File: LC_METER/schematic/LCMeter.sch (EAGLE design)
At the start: 164 parts, among them IC1 74HC595, IC2 74HC595, IC3 74HC595, IC4 74HC595, IC5 74HC595, IC6 MEGA8535, J10 0, J11 0, J123 0, J2 0, J3 0, J4 0, J5 0, J6 0, J7 0, J8 0, J9 0, Q2 12MHz, T1 BC847, T2 BC847, T3 BC857, T4 BC857, T5 BC847, T6 BC847, T7 BC847, U15 LM324, X1 C_X, X4 L_X, X5 USB_B, X6 USB_MICRO

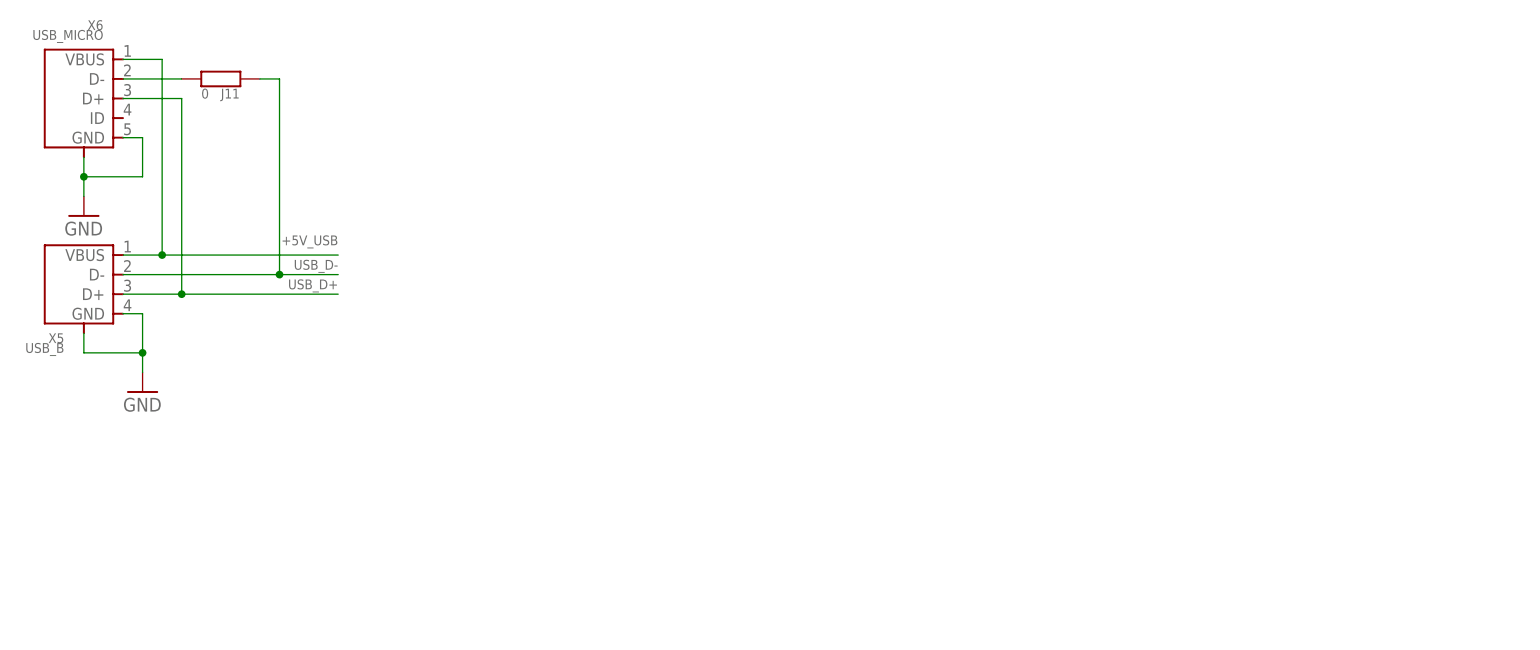
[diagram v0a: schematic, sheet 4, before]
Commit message: LCMeter Another changes
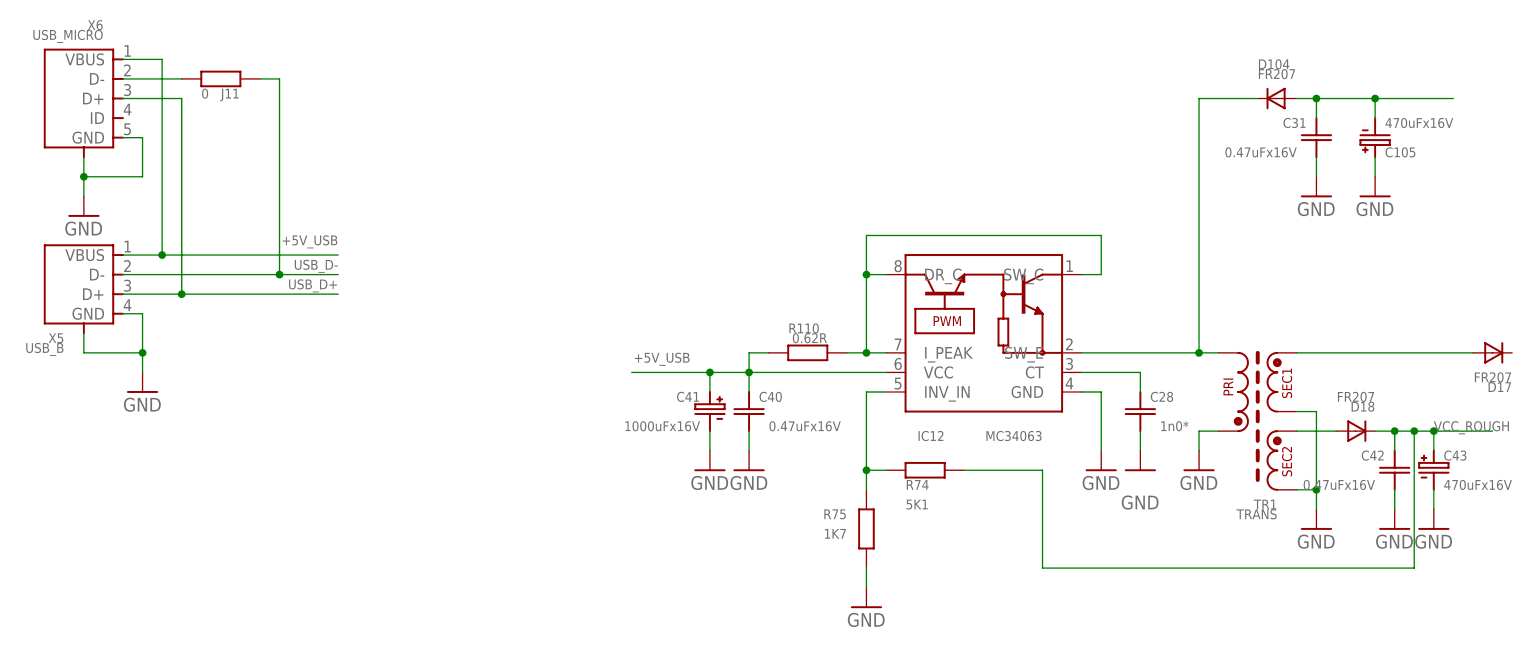
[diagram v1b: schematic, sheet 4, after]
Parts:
- added C105, C43: 470uFx16V, __MyCommonLib1:CE10MM
- added C28: 1n0*, __MyCommonLib1:CSMD_0805
- added C31, C40, C42: 0.47uFx16V, __MyCommonLib1:CSMD_0805
- added C41: 1000uFx16V, __MyCommonLib1:CE10MM
- added D104, D17, D18: FR207, __MyCommonLib1:1N4001DO-41_10MM
- added IC12: MC34063, __MyCommonLib1:MC34063(SO-8)
- added R110: 0.62R, __MyCommonLib1:RSMD_1206_BIG_GAP
- added R74: 5K1, __MyCommonLib1:RSMD_1206_BIG_GAP
- added R75: 1K7, __MyCommonLib1:RSMD_1206_BIG_GAP
- added TR1: TRANS, __MyCommonLib1:TRANS_3WINDRING25X10_HOR
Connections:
- new net N$10: D104.CATHODE, IC12.SW_E, TR1.PRI_END
- new net N$133: IC12.DR_C, IC12.I_PEAK, IC12.SW_C, R110.PIN1
- new net N$135: C28.PIN1, IC12.CT
- new net N$136: D18.ANODE, TR1.SEC2_START
- new net N$137: C105.-, C31.PIN1, D104.ANODE
- new net N$138: D17.ANODE, TR1.SEC1_START
- new net N$139: IC12.INV_IN, R74.PIN0, R75.PIN1
- net +5V_USB: now also C40.PIN1, C41.+, IC12.VCC, R110.PIN0
- net GND: now also C105.+, C28.PIN0, C31.PIN0, C40.PIN0, C41.-, C42.PIN0, C43.-, IC12.GND, R75.PIN0, TR1.PRI_START, TR1.SEC1_END, TR1.SEC2_END
- net VCC_ROUGH: now also C42.PIN1, C43.+, D18.CATHODE, R74.PIN1
